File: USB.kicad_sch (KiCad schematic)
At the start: 6 parts, among them J401 USB_C_Receptacle_USB2.0_16P, U402 TS3USB30ERSWR, U404 IP4234CZ6,115

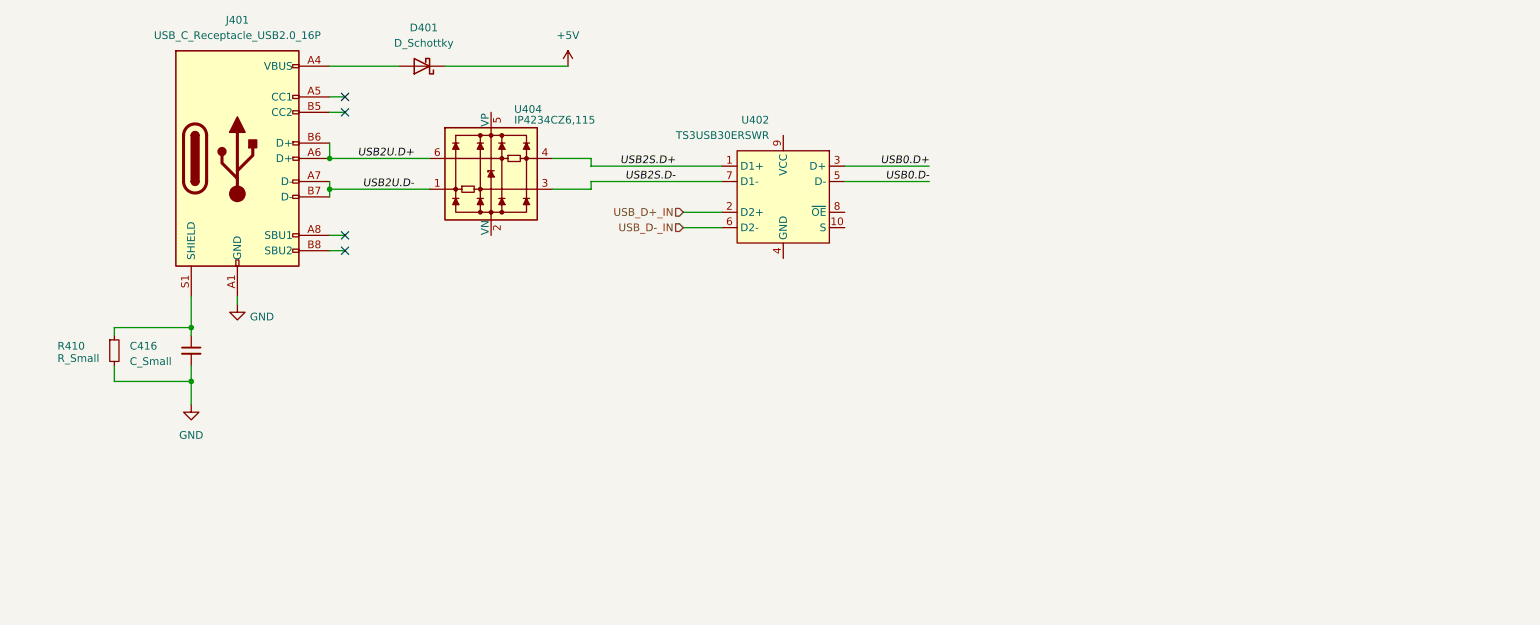
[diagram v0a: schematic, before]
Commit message: [3] Add USB power + data schematic
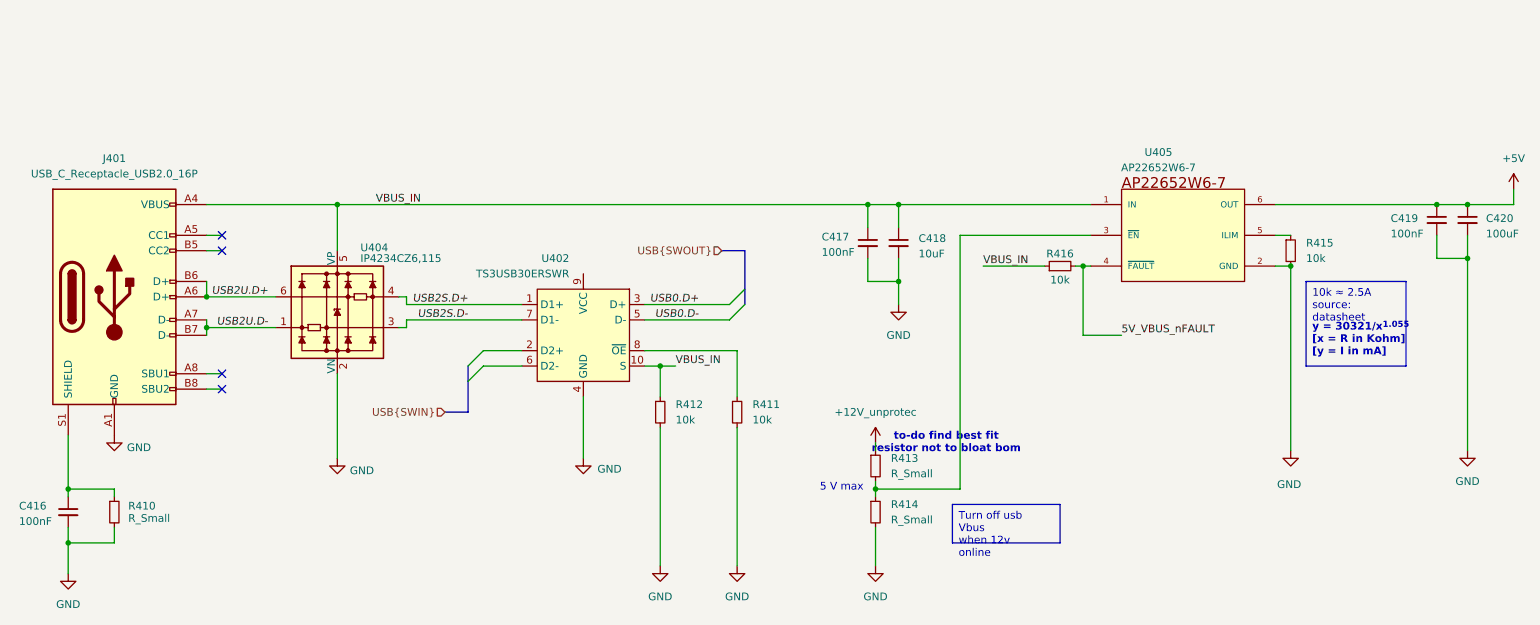
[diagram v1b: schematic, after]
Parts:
- removed D401: D_Schottky, symbol Device:D_Schottky
- added C417, C419: 100nF, symbol Device:C_Small
- added C418: 10uF, symbol Device:C_Small
- added C420: 100uF, symbol Device:C_Small
- added R411, R412: 10k, Resistor_SMD:R_0402_1005Metric, symbol Device:R_Small
- added R413, R414: R_Small, symbol Device:R_Small
- added R415, R416: 10k, symbol Device:R_Small
- added U405: AP22652W6-7, AP22652W6-7:SOT-26, symbol AP22652W6-7:AP22652W6-7
- C416: value C_Small -> 100nF
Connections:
- net +5V: now also C419.1, C420.1, U405.6 (OUT)
- net GND: now also U402.4 (GND), U404.2 (VN), C417.2, C418.2, C419.2, C420.2, R411.2, R412.2, R414.2, R415.2, U405.2 (GND)
- net VBUS_IN: now reaches U402.10 (S)
- net VBUS_IN: now also J401.A4 (VBUS), J401.A9 (VBUS), J401.B4 (VBUS), J401.B9 (VBUS), U404.5 (VP), C417.1, C418.1, R412.1, R416.1, U405.1 (IN)
- net at U402.8 (~{OE}): now also R411.1
- net USB_D+_IN: no longer names the net of U402.2 (D2+)
- net USB_D-_IN: no longer names the net of U402.6 (D2-)
- new net: R413.2, R414.1, U405.3 (~{EN})
- new net: R415.1, U405.5 (ILIM)
- new net +12V_unprotec: R413.1
- new net 5V_VBUS_nFAULT: R416.2, U405.4 (~{FAULT})
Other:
- note added: "5 V max"
- note added: "to-do find best fit resistor not to bloat bom"
- note added: "y = 30321/x^{1.055} [x = R in Kohm] [y = I in mA]"
- company: (none) -> ModuCard System
- title: (none) -> USB type C
- moved on the sheet: C416, J401, R410, U402, U404

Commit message: [3] Fix schematic sheet descriptions
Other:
- company: ModuCard System -> KoNaR
- title: USB type C -> ModuCard base module
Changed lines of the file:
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@@
 	(paper "A4")
 	(title_block
-		(title "USB type C")
-		(company "ModuCard System")
+		(title "ModuCard base module")
+		(date "2024-12-23")
+		(rev "1.0.0")
+		(company "KoNaR")
 		(comment 1 "Base project authors: Dominik Pluta, Artem Horiunov")
 		(comment 2 "Project author: <author>")
@@
 		)
 		(instances
-			(project ""
+			(project "base-module"
 				(path "/090a8e41-87a8-4fb1-998b-60a2c0dc4cee/8fd5ae83-0658-4178-9e81-18085647e2bb"
 					(reference "U402")
@@
 		)
 		(instances
-			(project ""
+			(project "base-module"
 				(path "/090a8e41-87a8-4fb1-998b-60a2c0dc4cee/8fd5ae83-0658-4178-9e81-18085647e2bb"
 					(reference "U405")
@@
 		)
 		(instances
-			(project ""
+			(project "base-module"
 				(path "/090a8e41-87a8-4fb1-998b-60a2c0dc4cee/8fd5ae83-0658-4178-9e81-18085647e2bb"
 					(reference "#PWR0428")
@@
 		)
 		(instances
-			(project ""
+			(project "base-module"
 				(path "/090a8e41-87a8-4fb1-998b-60a2c0dc4cee/8fd5ae83-0658-4178-9e81-18085647e2bb"
 					(reference "#PWR0425")
@@
 		)
 		(instances
-			(project ""
+			(project "base-module"
 				(path "/090a8e41-87a8-4fb1-998b-60a2c0dc4cee/8fd5ae83-0658-4178-9e81-18085647e2bb"
 					(reference "C416")
@@
 		)
 		(instances
-			(project ""
+			(project "base-module"
 				(path "/090a8e41-87a8-4fb1-998b-60a2c0dc4cee/8fd5ae83-0658-4178-9e81-18085647e2bb"
 					(reference "R410")
@@
 		)
 		(instances
-			(project ""
+			(project "base-module"
 				(path "/090a8e41-87a8-4fb1-998b-60a2c0dc4cee/8fd5ae83-0658-4178-9e81-18085647e2bb"
 					(reference "U404")
@@
 		)
 		(instances
-			(project ""
+			(project "base-module"
 				(path "/090a8e41-87a8-4fb1-998b-60a2c0dc4cee/8fd5ae83-0658-4178-9e81-18085647e2bb"
 					(reference "#PWR0434")
@@
 		)
 		(instances
-			(project ""
+			(project "base-module"
 				(path "/090a8e41-87a8-4fb1-998b-60a2c0dc4cee/8fd5ae83-0658-4178-9e81-18085647e2bb"
 					(reference "J401")
@@
 		)
 		(instances
-			(project ""
+			(project "base-module"
 				(path "/090a8e41-87a8-4fb1-998b-60a2c0dc4cee/8fd5ae83-0658-4178-9e81-18085647e2bb"
 					(reference "R413")
@@
 		)
 		(instances
-			(project ""
+			(project "base-module"
 				(path "/090a8e41-87a8-4fb1-998b-60a2c0dc4cee/8fd5ae83-0658-4178-9e81-18085647e2bb"
 					(reference "R411")
@@
 		)
 		(instances
-			(project ""
+			(project "base-module"
 				(path "/090a8e41-87a8-4fb1-998b-60a2c0dc4cee/8fd5ae83-0658-4178-9e81-18085647e2bb"
 					(reference "#PWR0437")

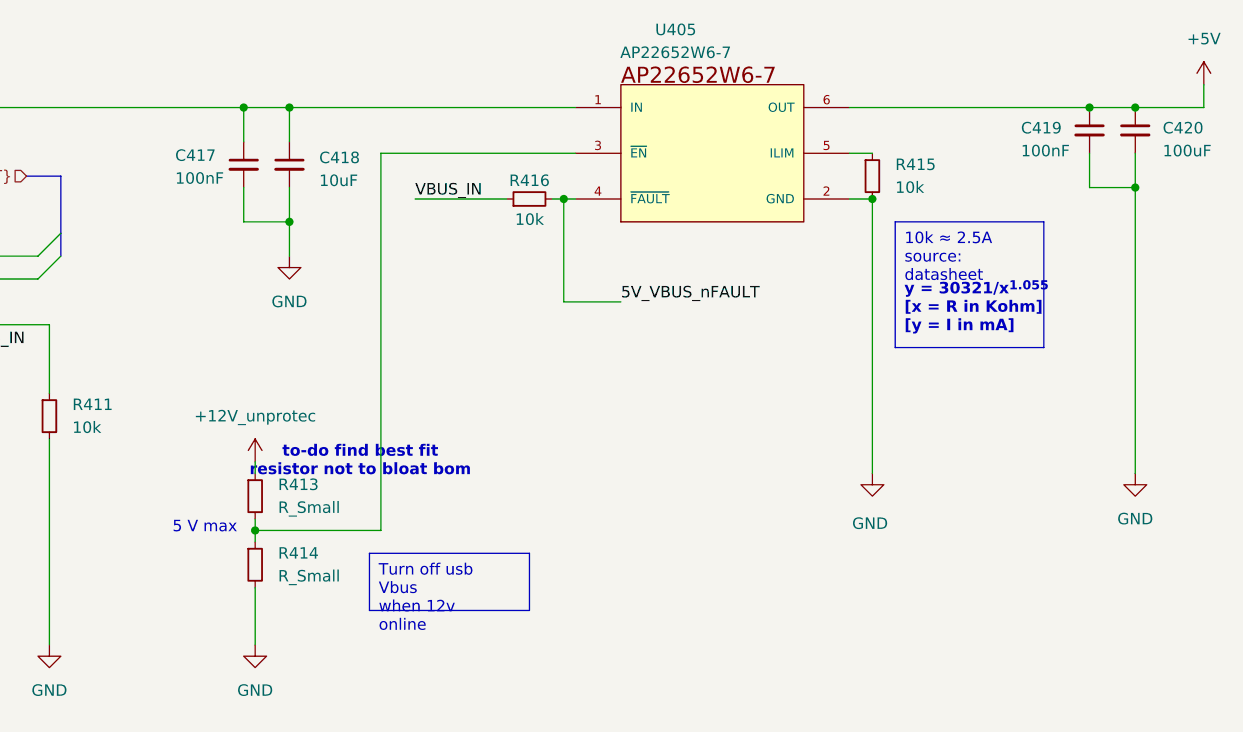
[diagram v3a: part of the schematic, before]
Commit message: [3] Delete USB power switch
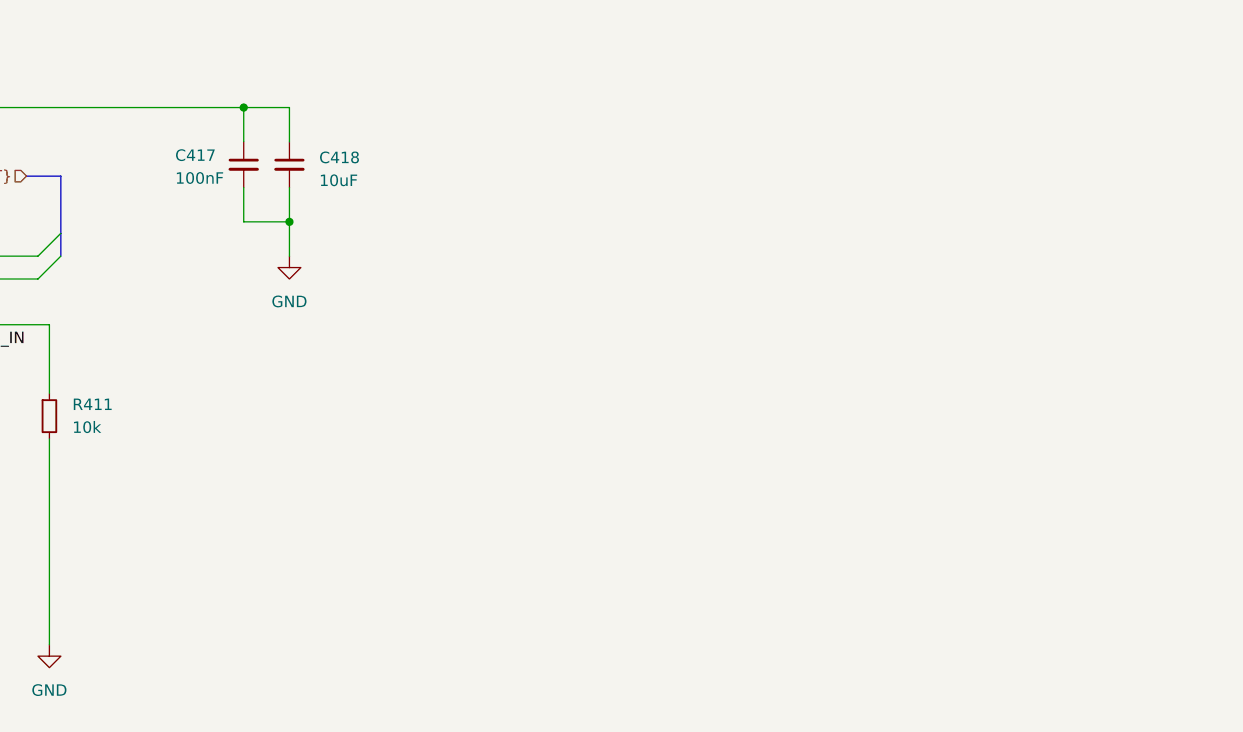
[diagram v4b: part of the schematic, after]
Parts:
- removed C419: 100nF, symbol Device:C_Small
- removed C420: 100uF, symbol Device:C_Small
- removed R413, R414: R_Small, symbol Device:R_Small
- removed R415, R416: 10k, symbol Device:R_Small
- removed U405: AP22652W6-7, AP22652W6-7:SOT-26, symbol AP22652W6-7:AP22652W6-7
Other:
- note removed: "5 V max"
- note removed: "to-do find best fit resistor not to bloat bom"
- note removed: "y = 30321/x^{1.055} [x = R in Kohm] [y = I in mA]"

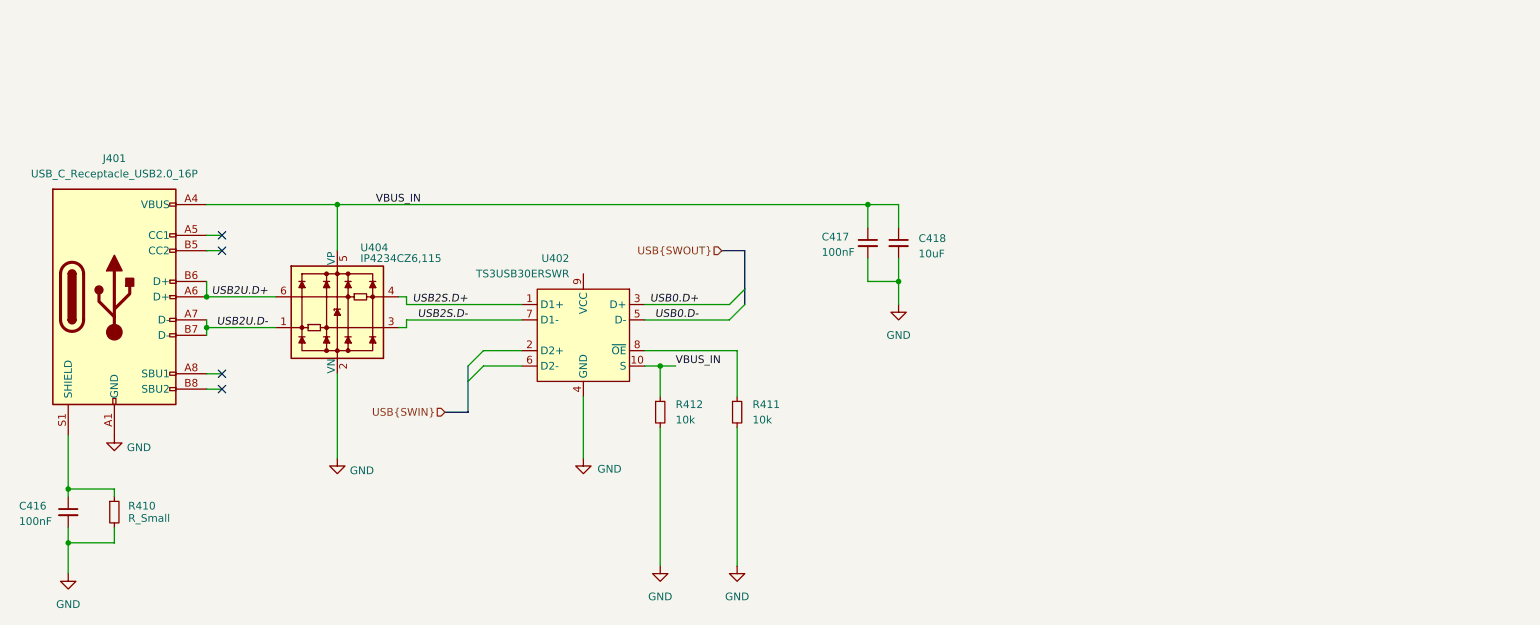
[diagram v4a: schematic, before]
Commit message: [3] Fix schematic typos
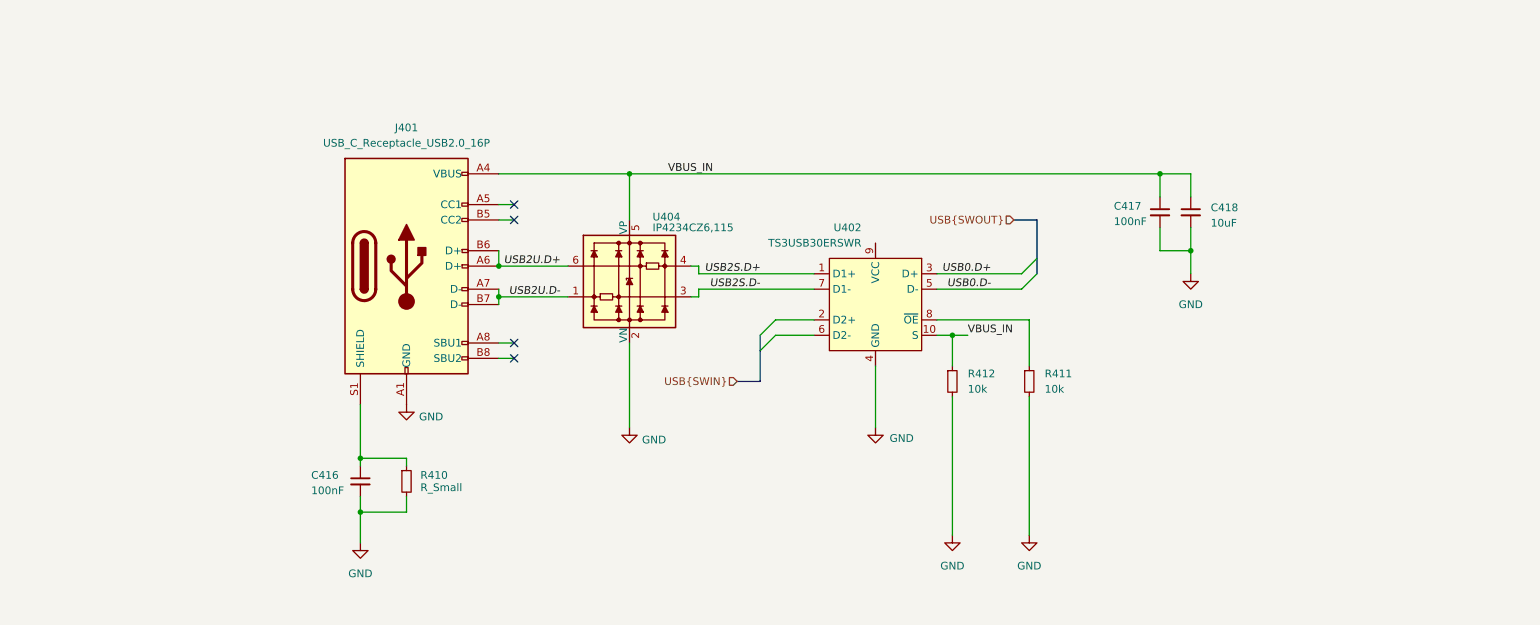
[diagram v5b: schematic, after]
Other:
- moved on the sheet: C416, C417, C418, J401, R410, R411, R412, U402, U404
